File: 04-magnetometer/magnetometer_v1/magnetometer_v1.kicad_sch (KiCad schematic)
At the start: 38 parts, among them IC1 STM32F072CBT6, IC2 TMAG5170A1QDGKR, IC3 TCAN1042GVDRQ1, J1 Conn_02x04_Odd_Even, J2 USB4110-GF-A, SW1 SW_Push, SW2 SW_Push, SW3 SW_SPDT, U1 SPX3819M5-L-3-3/TR

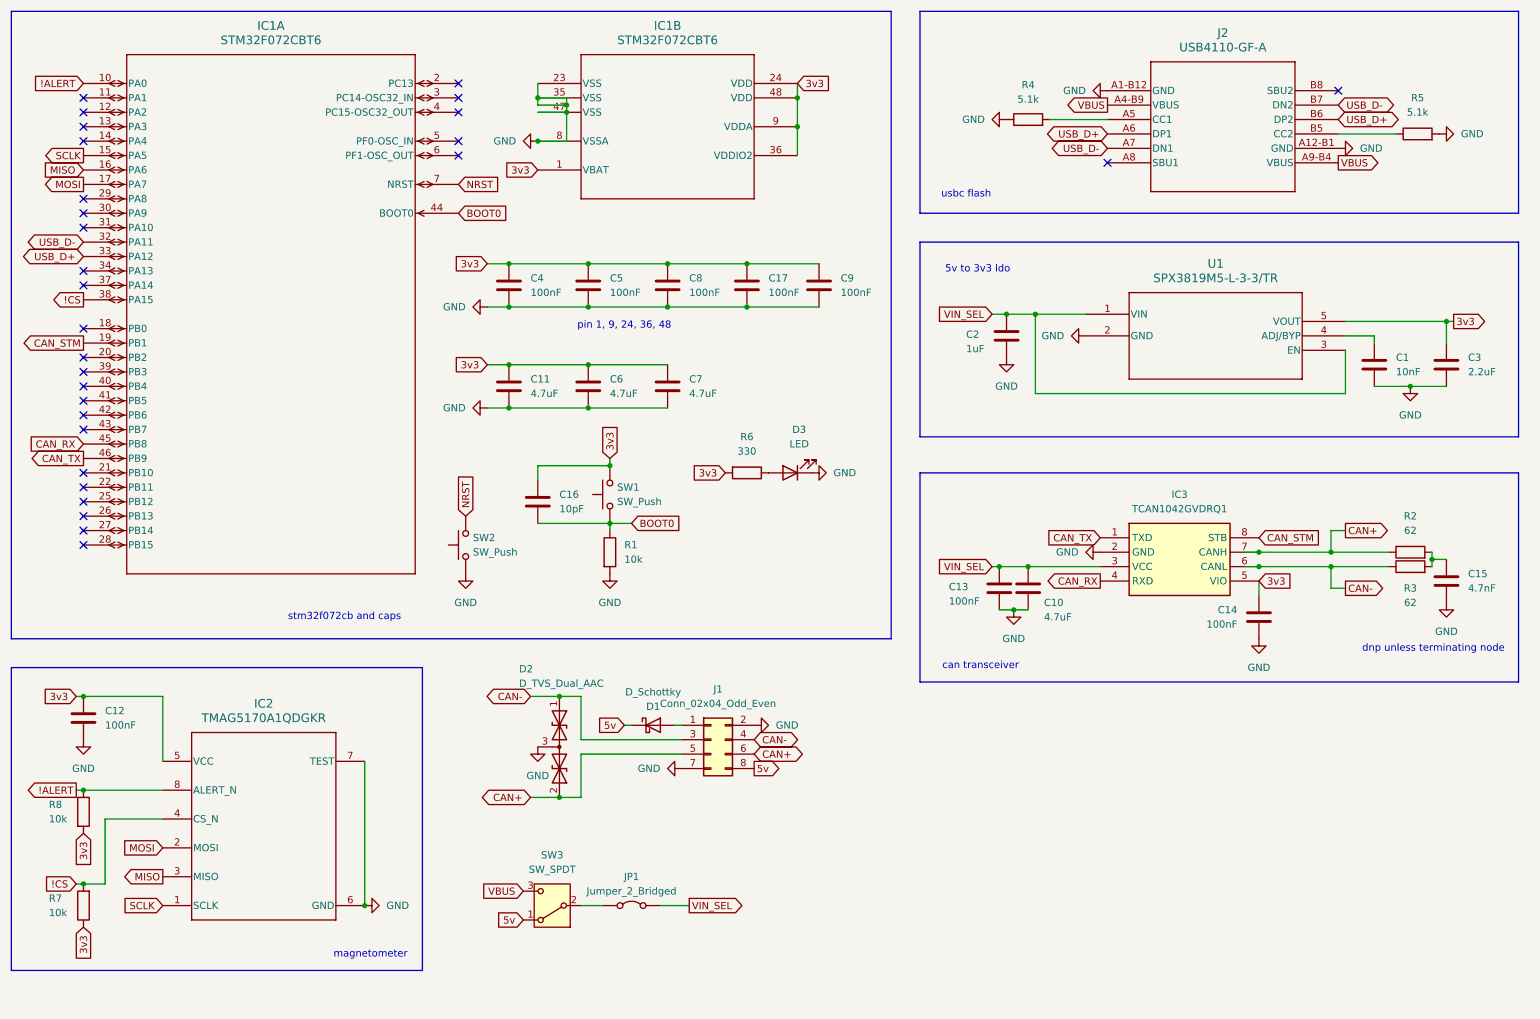
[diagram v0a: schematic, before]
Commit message: preliminary routing
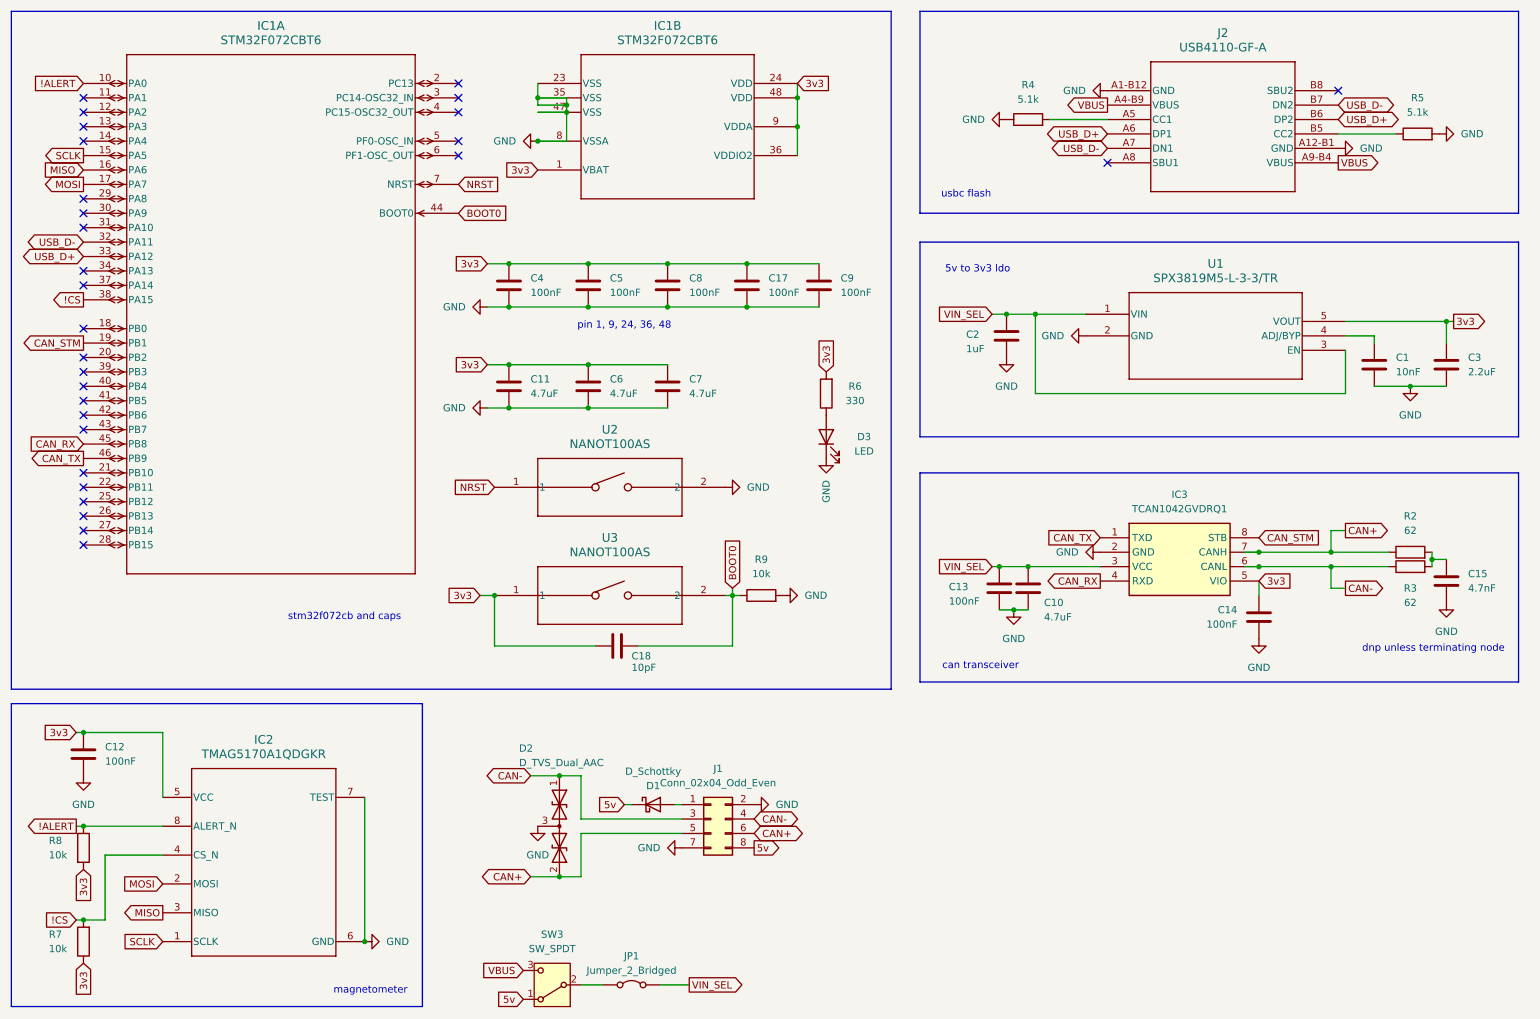
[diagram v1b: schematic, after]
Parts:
- removed C16: 10pF, Capacitor_SMD:C_0402_1005Metric, symbol Device:C
- removed R1: 10k, Resistor_SMD:R_0402_1005Metric, symbol Device:R
- removed SW1, SW2: SW_Push, mag-fp:SW_NANOT-AS_CNK, symbol Switch:SW_Push
- added C18: 10pF, Capacitor_SMD:C_0402_1005Metric, symbol Device:C
- added R9: 10k, Resistor_SMD:R_0402_1005Metric, symbol Device:R
- added U2, U3: NANOT100AS, mag-fp:SW_NANOT-AS_CNK, symbol mag-symbols:NANOT100AS
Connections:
- net 3v3: now also C18.2, U3.1
- net BOOT0: now also C18.1, R9.1, U3.2
- net GND: now also R9.2, U2.2
- net NRST: now also U2.1
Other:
- moved on the sheet: C12, D1, D2, D3, IC2, J1, JP1, R6, R7, R8, SW3
